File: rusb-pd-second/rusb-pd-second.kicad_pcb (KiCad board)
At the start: 2 copper layers, 25.5 x 24.6 mm, 18 parts, among them J1 Conn_02x05_Counter_Clockwise, J2 Conn_01x02, U1 AMS1117-3.3, U3 FUSB302BMPX, U4 CH32V003FxUx

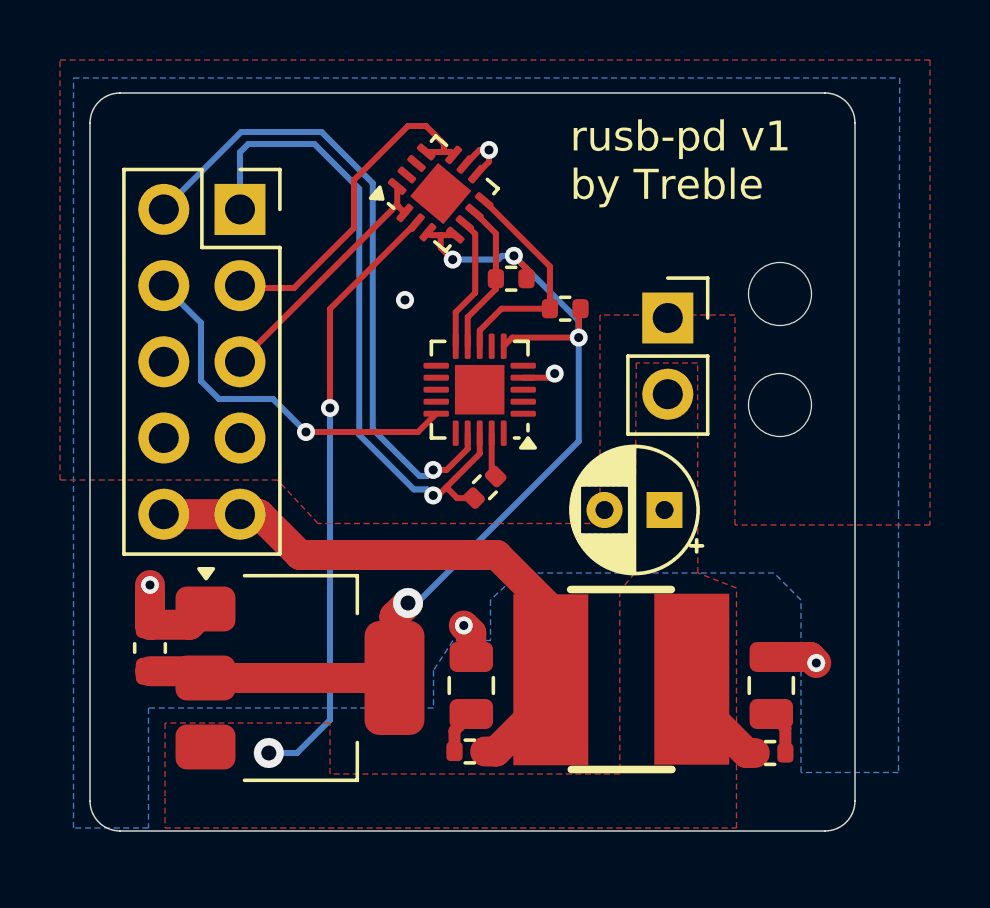
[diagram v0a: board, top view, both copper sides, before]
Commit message: lotta changes (described in the articel)
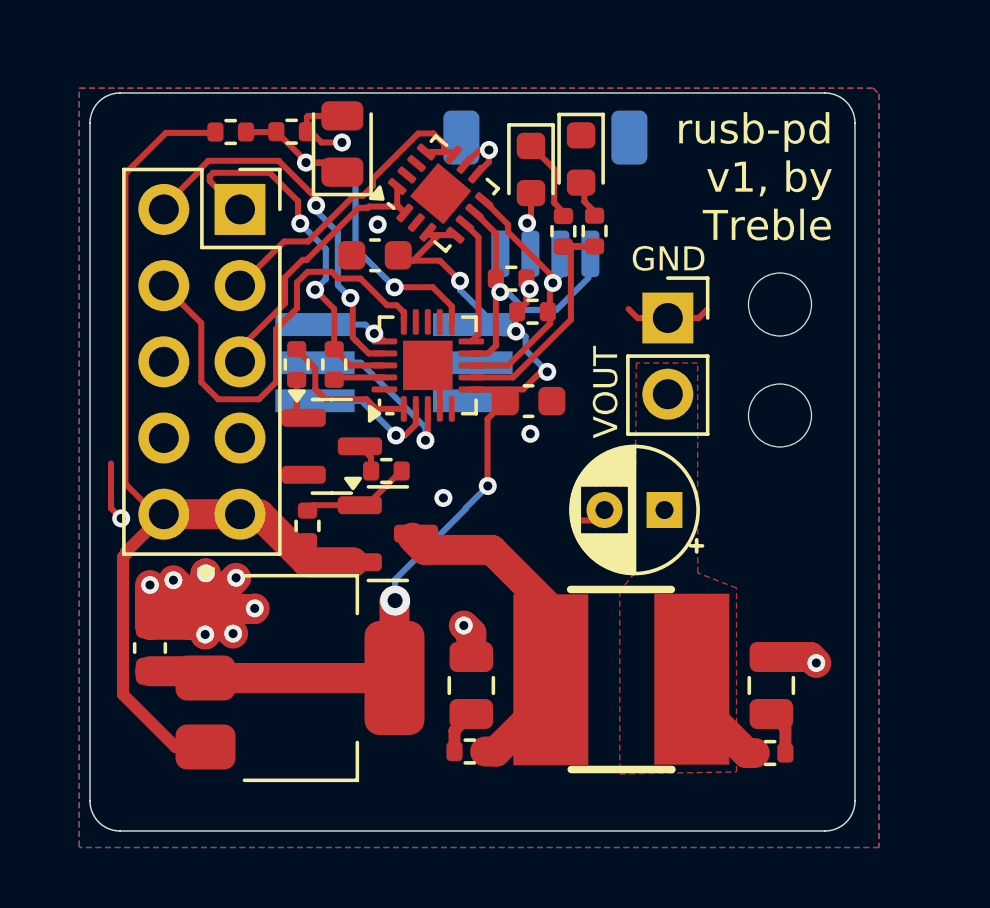
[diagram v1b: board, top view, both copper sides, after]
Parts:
- removed the G*** at (153.8, 119.6)
- added C5: 100n, Capacitor_SMD:C_0603_1608Metric, F.Cu at (143.0, 105.5)
- added C6: 100n, Capacitor_SMD:C_0603_1608Metric, F.Cu at (148.1, 110.4)
- added D1: 3V6, Diode_SMD:D_0805_2012Metric, F.Cu at (141.9, 101.8)
- added D2: LED1, LED_SMD:LED_0603_1608Metric, F.Cu at (149.9, 102.3)
- added D3: LED2, LED_SMD:LED_0603_1608Metric, F.Cu at (148.2, 102.7)
- added G***: LOGO, rusb-pd-second:frieren_4, B.Cu at (145.6, 116.8)
- added J3: qwiic, Connector_JST:JST_SH_SM04B-SRSS-TB_1x04-1MP_P1.00mm_Horizontal, B.Cu at (148.7, 103.5)
- added Q1: AO3401, Package_TO_SOT_SMD:SOT-23, F.Cu at (143.4, 114.8)
- added Q2: BC847, Package_TO_SOT_SMD:SOT-23, F.Cu at (141.6, 111.9)
- added R10: 1K5, Resistor_SMD:R_0402_1005Metric, F.Cu at (140.4, 109.2)
- added R11: 5.1K, Resistor_SMD:R_0402_1005Metric, F.Cu at (150.3, 104.7)
- added R12: 5.1K, Resistor_SMD:R_0402_1005Metric, F.Cu at (149.3, 104.7)
- added R3: 1K5, Resistor_SMD:R_0402_1005Metric, F.Cu at (140.2, 101.4)
- added R4: 15K, Resistor_SMD:R_0402_1005Metric, F.Cu at (138.2, 101.4)
- added R8: 1K5, Resistor_SMD:R_0402_1005Metric, F.Cu at (140.8, 114.5)
- added R9: 4K7, Resistor_SMD:R_0402_1005Metric, F.Cu at (143.4, 112.7)
- added SW1: SW_DIP_x03, rusb-pd-second:SW-SMD_6P-P1.27_EU-03KS, B.Cu at (143.6, 109.1)
- R1, R2: value 3K3 -> 1K5
- moved R5 6.48 mm to (141.6, 109.2), turned to 90 degrees
- moved U4 1.91 mm to (144.8, 109.2), turned to 90 degrees
- moved R1 1.09 mm to (148.2, 107.4), turned to 180 degrees
- moved REF** 0.35 mm to (156.5, 107.2)
- moved REF** 0.35 mm to (156.5, 110.8)
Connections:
- L1 pad 1: /TYPEC_VBUS -> Net-(Q1-D)
- R7 pad 2: /TYPEC_VBUS -> Net-(Q1-D)
- U1 pad 3: VBUS -> /TYPEC_VBUS
- U3 pad 2: VBUS -> unconnected-(U3-VBUS-Pad2)
- U4 pad 1: unconnected-(U4-PD7-Pad1) -> /VBUS_EN
- U4 pad 11: unconnected-(U4-PC4-Pad11) -> /VBUS_ADC
- U4 pad 16: unconnected-(U4-PD2-Pad16) -> /CFG3
- U4 pad 2: unconnected-(U4-PA1-Pad2) -> /CFG1
- U4 pad 21: (no net) -> GND
- U4 pad 3: unconnected-(U4-PA2-Pad3) -> /CFG2
- U4 pad 7: unconnected-(U4-PC0-Pad7) -> /LED
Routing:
- net VBUS: track 23.8 -> 3.49 mm, vias 2 -> 0
- net GND: track 9.21 -> 27.5 mm, vias 6 -> 15
- net /VBUS_ADC: track 0.00 -> 12.6 mm, vias 0 -> 2
- net /TYPEC_VBUS: track 20.1 -> 32.6 mm
- net Net-(Q1-D): track 0.00 -> 11.5 mm
- net /D-: track 21.8 -> 12.6 mm, vias 1 -> 2
- net /D+: track 21.6 -> 12.8 mm, vias 1 -> 2
- net /LED: track 0.00 -> 8.53 mm
- net /CFG2: track 0.00 -> 6.09 mm, vias 0 -> 1
- net /VBUS_EN: track 0.00 -> 4.80 mm
- net /CFG1: track 0.00 -> 4.51 mm, vias 0 -> 1
- net /F_SCL: track 5.15 -> 9.30 mm, vias 0 -> 1
- net Net-(Q1-G): track 0.00 -> 3.78 mm
- net Net-(D3-K): track 0.00 -> 2.82 mm
- net /CFG3: track 0.00 -> 2.54 mm, vias 0 -> 1
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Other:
- board text added: "GND"
- board text added: "VOUT"
- board text added: "gnd vcc sda scl"
- board text added: "rusb-pd v1, by Treble"
- board text removed: "rusb-pd v1 by Treble"
